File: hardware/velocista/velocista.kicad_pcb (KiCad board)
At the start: 2 copper layers, 120 x 106.2 mm, 19 parts, among them J1 XT30, J2 Cable_PAD, J3 Cable_PAD, J4 QTR8a, SW1 SW_Push, SW3 SW_SPDT, U1 TB6612FNG, U2 Mini360, U4 ESP32-DEVKITC-32D

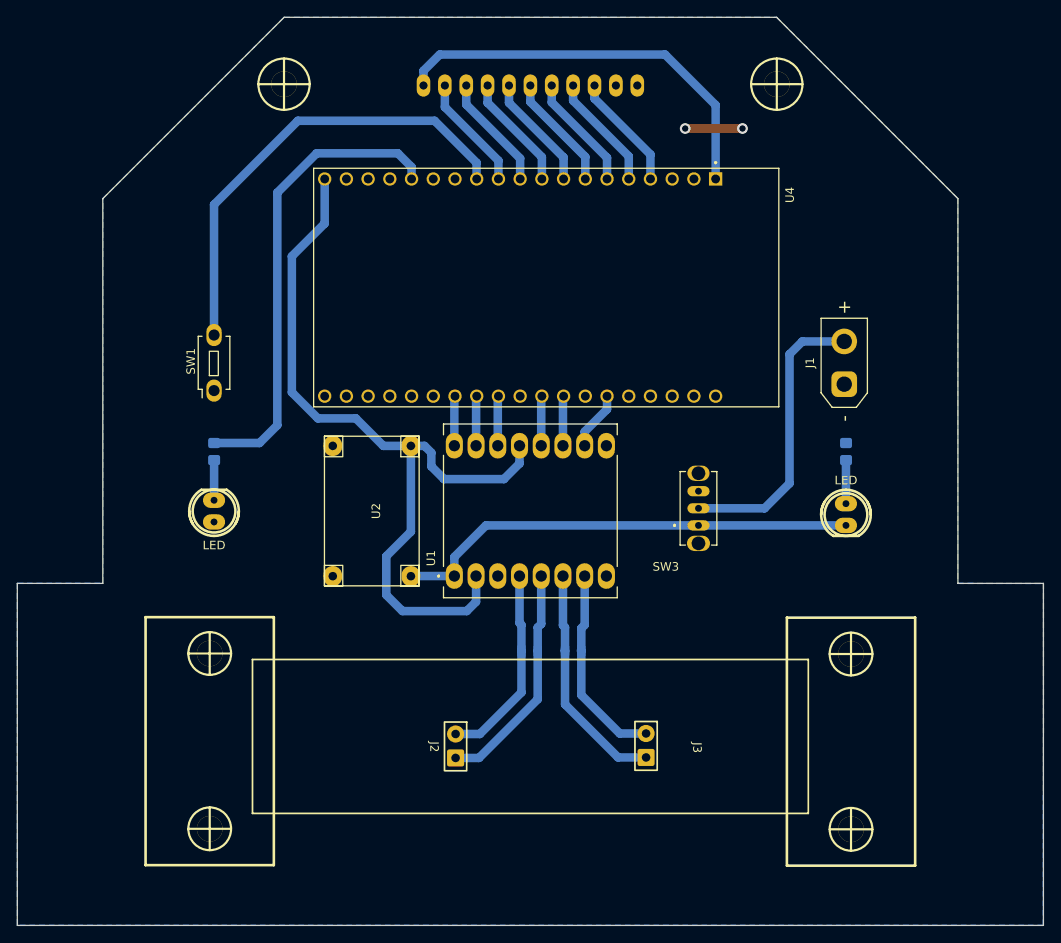
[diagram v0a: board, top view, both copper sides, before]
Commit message: act placa
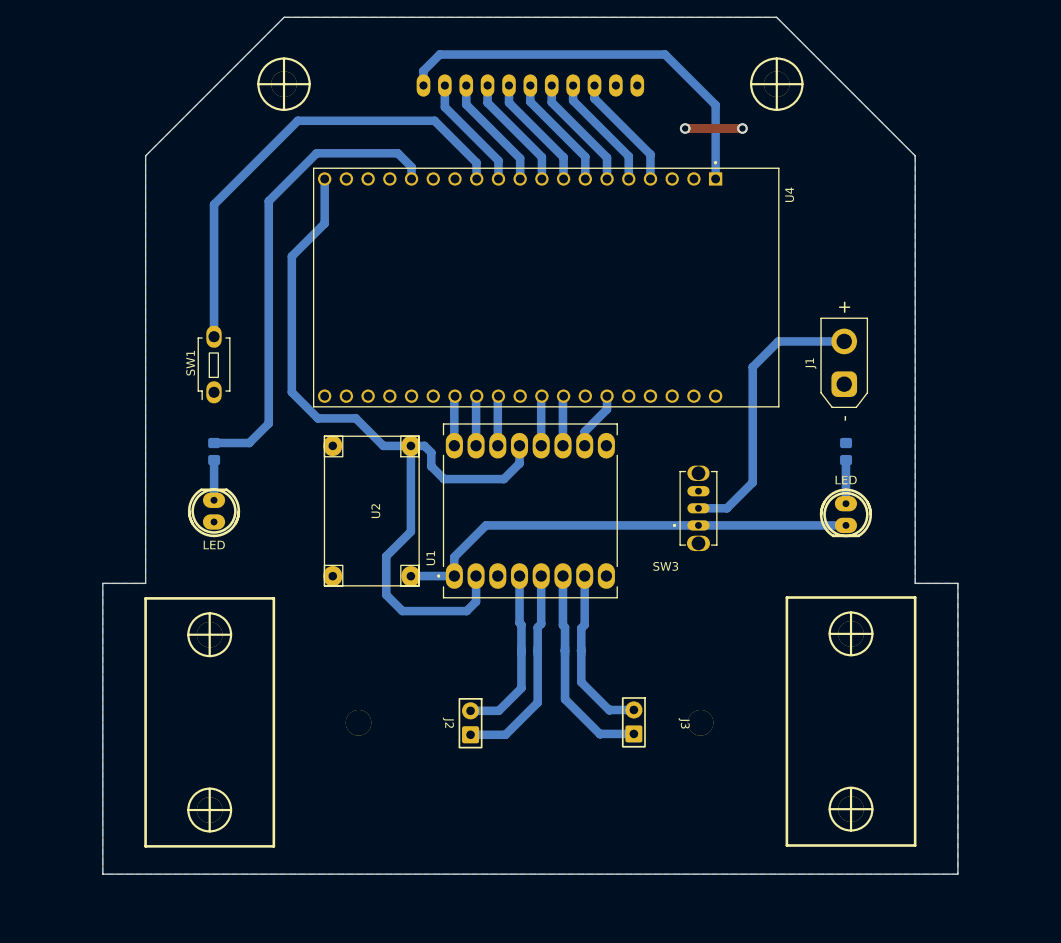
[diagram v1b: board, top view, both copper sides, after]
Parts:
- added ?: , , F.Cu at (130.2, 117.0)
- added ?: , , F.Cu at (90.2, 117.0)
- moved J2 3.23 mm to (100.3, 117.1)
- moved J3 3.10 mm to (119.4, 117.0)
- moved Pololu_Micro_Gear_Motor 2.36 mm to (147.8, 116.8)
- moved Pololu_Micro_Gear_Motor 2.20 mm to (72.8, 117.0)
- moved SW1 0.20 mm to (73.3, 78.3)
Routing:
- net Net-(U1-B01): track 23.6 -> 20.2 mm
- net Net-(U1-A01): track 23.4 -> 20.3 mm
- net Net-(U1-B02): track 27.2 -> 24.3 mm
- net Net-(U1-A02): track 27.0 -> 24.4 mm
- net Net-(J1-Pin_2): track 34.0 -> 33.0 mm
- net LED: track 55.1 -> 54.4 mm
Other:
- board size 120 x 106.2 mm -> 100 x 100.2 mm
